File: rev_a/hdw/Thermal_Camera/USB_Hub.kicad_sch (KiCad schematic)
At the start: 28 parts

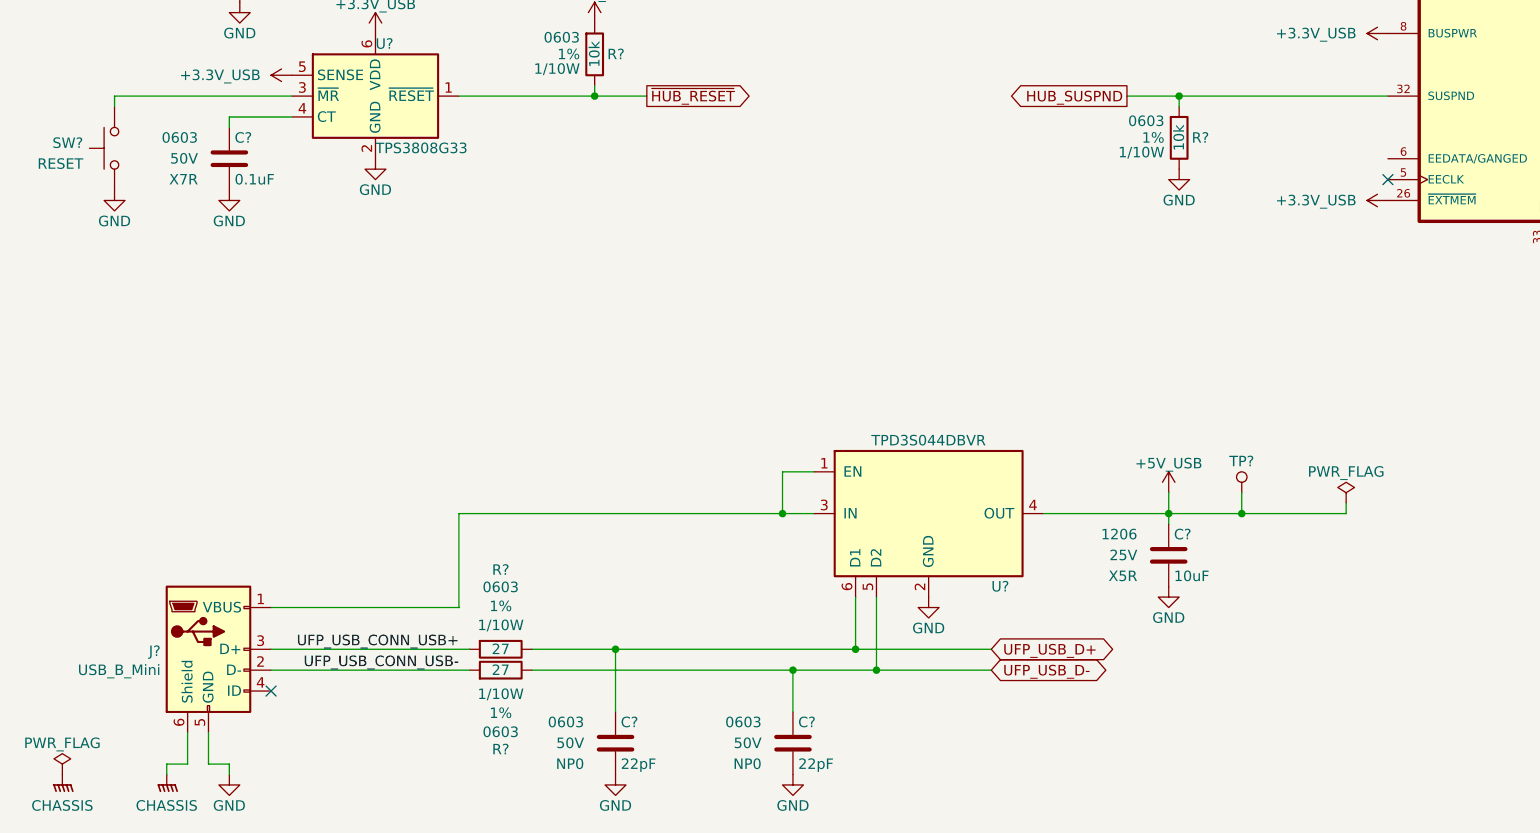
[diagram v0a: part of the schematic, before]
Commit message: added some more USB stuff
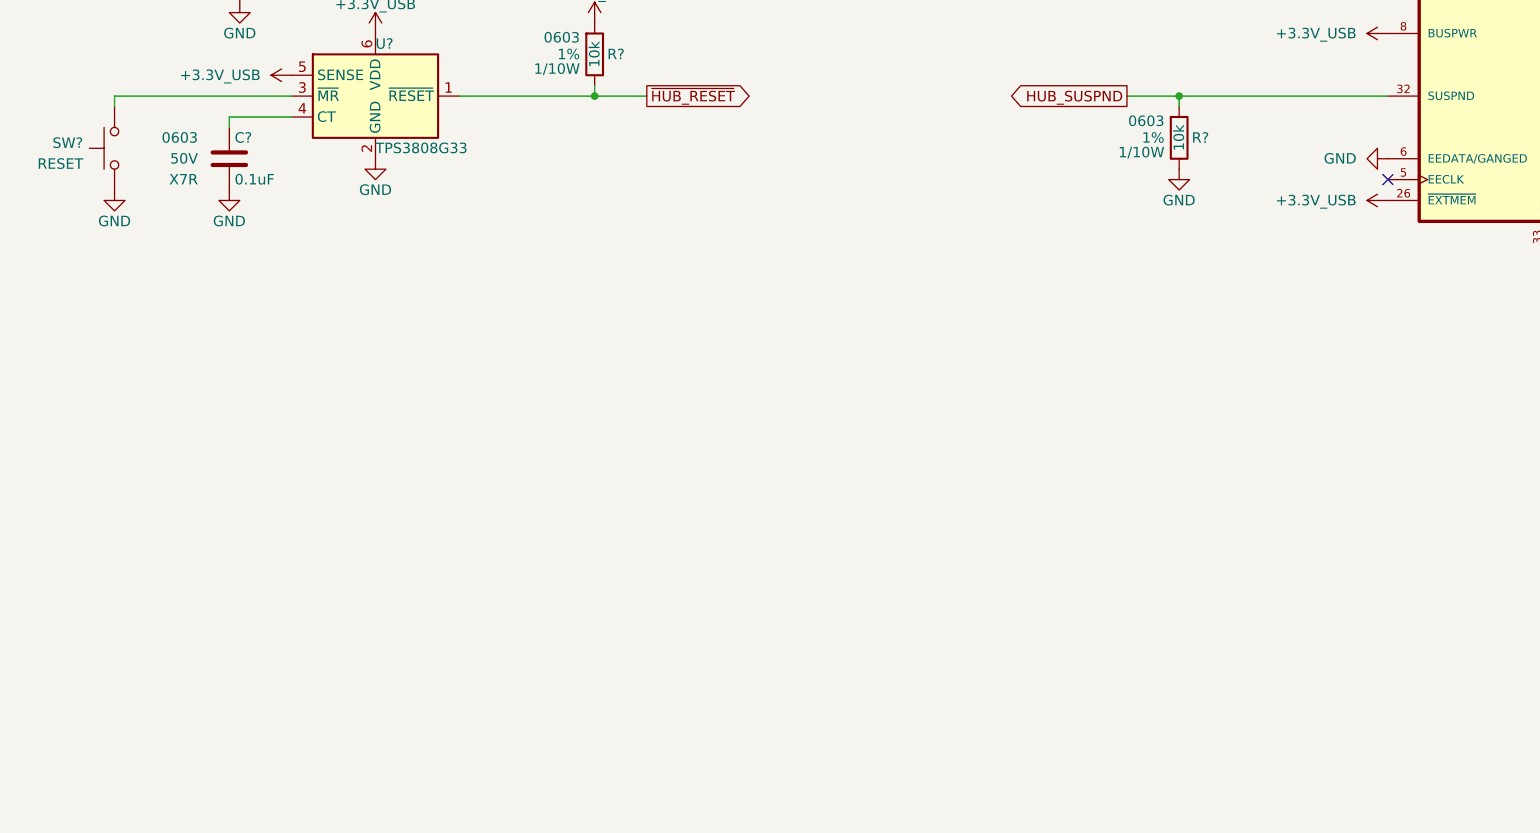
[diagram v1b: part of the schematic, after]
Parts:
- removed C?: 10uF, Capacitors_SMD:C_1206, symbol Custom_Library:C_Custom
- removed C? (x2): 22pF, Capacitors_SMD:C_0603, symbol Custom_Library:C_Custom
- removed J?: USB_B_Mini, Connectors:USB_Mini-B, symbol Connector:USB_B_Mini
- removed R? (x2): 27, Resistors_SMD:R_0603, symbol Custom_Library:R_Custom
- removed TP?: TP, Custom Footprints Library:Test_Point, symbol Custom_Library:TP
- removed U?: TPD3S044DBVR, TO_SOT_Packages_SMD:SOT-23-6, symbol Custom_Library:TPD3S014DBVR
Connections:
- net GND: now also U?.6 (EEDATA/GANGED)
- no-connect marks 11 -> 10
